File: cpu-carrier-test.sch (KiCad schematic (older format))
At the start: 6 parts, among them SW1 SW_Push

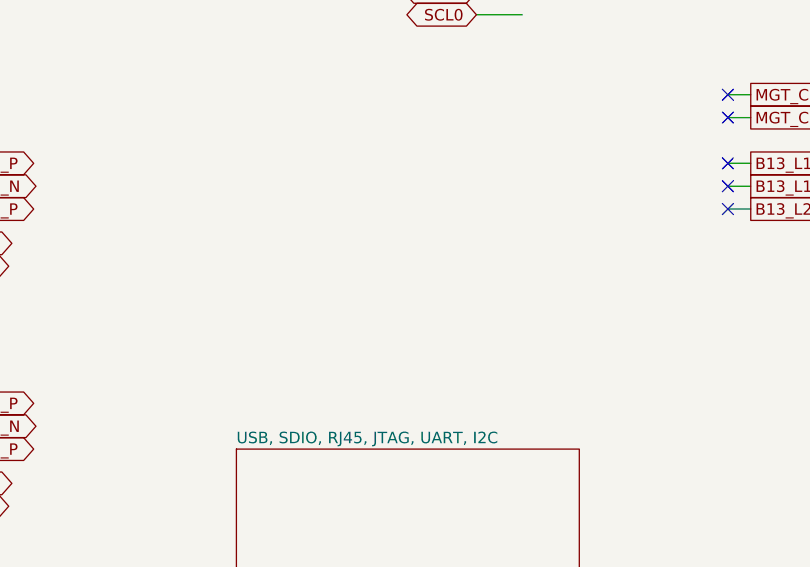
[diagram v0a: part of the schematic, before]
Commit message: don't remember changes :-(
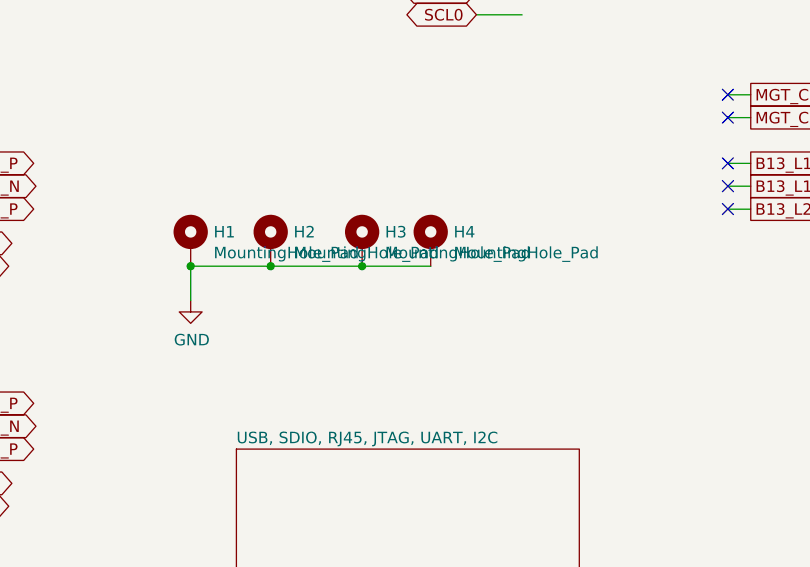
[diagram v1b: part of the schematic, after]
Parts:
- added H1, H2, H3, H4: MountingHole_Pad, MountingHole:MountingHole_3.2mm_M3_ISO14580_Pad_TopBottom, symbol Mechanical:MountingHole_Pad
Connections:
- wire segments 80 -> 84
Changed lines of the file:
@@
 	1    0    0    -1
 $EndComp
+$Comp
+L Mechanical:MountingHole_Pad H1
+U 1 1 60DE1513
+P 4050 4600
+F 0 "H1" H 4150 4649 50  0000 L CNN
+F 1 "MountingHole_Pad" H 4150 4558 50  0000 L CNN
+F 2 "MountingHole:MountingHole_3.2mm_M3_ISO14580_Pad_TopBottom" H 4050 4600 50  0001 C CNN
+F 3 "~" H 4050 4600 50  0001 C CNN
+	1    4050 4600
+	1    0    0    -1
+$EndComp
+$Comp
+L Mechanical:MountingHole_Pad H2
+U 1 1 60DE15CA
+P 4400 4600
+F 0 "H2" H 4500 4649 50  0000 L CNN
+F 1 "MountingHole_Pad" H 4500 4558 50  0000 L CNN
+F 2 "MountingHole:MountingHole_3.2mm_M3_ISO14580_Pad_TopBottom" H 4400 4600 50  0001 C CNN
+F 3 "~" H 4400 4600 50  0001 C CNN
+	1    4400 4600
+	1    0    0    -1
+$EndComp
+$Comp
+L Mechanical:MountingHole_Pad H3
+U 1 1 60DE1744
+P 4800 4600
+F 0 "H3" H 4900 4649 50  0000 L CNN
+F 1 "MountingHole_Pad" H 4900 4558 50  0000 L CNN
+F 2 "MountingHole:MountingHole_3.2mm_M3_ISO14580_Pad_TopBottom" H 4800 4600 50  0001 C CNN
+F 3 "~" H 4800 4600 50  0001 C CNN
+	1    4800 4600
+	1    0    0    -1
+$EndComp
+$Comp
+L Mechanical:MountingHole_Pad H4
+U 1 1 60DE197D
+P 5100 4600
+F 0 "H4" H 5200 4649 50  0000 L CNN
+F 1 "MountingHole_Pad" H 5200 4558 50  0000 L CNN
+F 2 "MountingHole:MountingHole_3.2mm_M3_ISO14580_Pad_TopBottom" H 5100 4600 50  0001 C CNN
+F 3 "~" H 5100 4600 50  0001 C CNN
+	1    5100 4600
+	1    0    0    -1
+$EndComp
+$Comp
+L power:GND #PWR?
+U 1 1 60DE1D1B
+P 4050 4850
+F 0 "#PWR?" H 4050 4600 50  0001 C CNN
+F 1 "GND" H 4055 4677 50  0000 C CNN
+F 2 "" H 4050 4850 50  0001 C CNN
+F 3 "" H 4050 4850 50  0001 C CNN
+	1    4050 4850
+	1    0    0    -1
+$EndComp
+Wire Wire Line
+	4050 4850 4050 4700
+Wire Wire Line
+	5100 4700 4800 4700
+Connection ~ 4050 4700
+Connection ~ 4400 4700
+Wire Wire Line
+	4400 4700 4050 4700
+Connection ~ 4800 4700
+Wire Wire Line
+	4800 4700 4400 4700
 $EndSCHEMATC
